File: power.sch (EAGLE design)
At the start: 29 parts, among them CN1 21700, CN2 21700, CN3 21700, CN5 15PIN 0.5MM, Q1 SIRA36DP-T1-GE3, Q2 SIRA36DP-T1-GE3, U1 MAX17320G20+

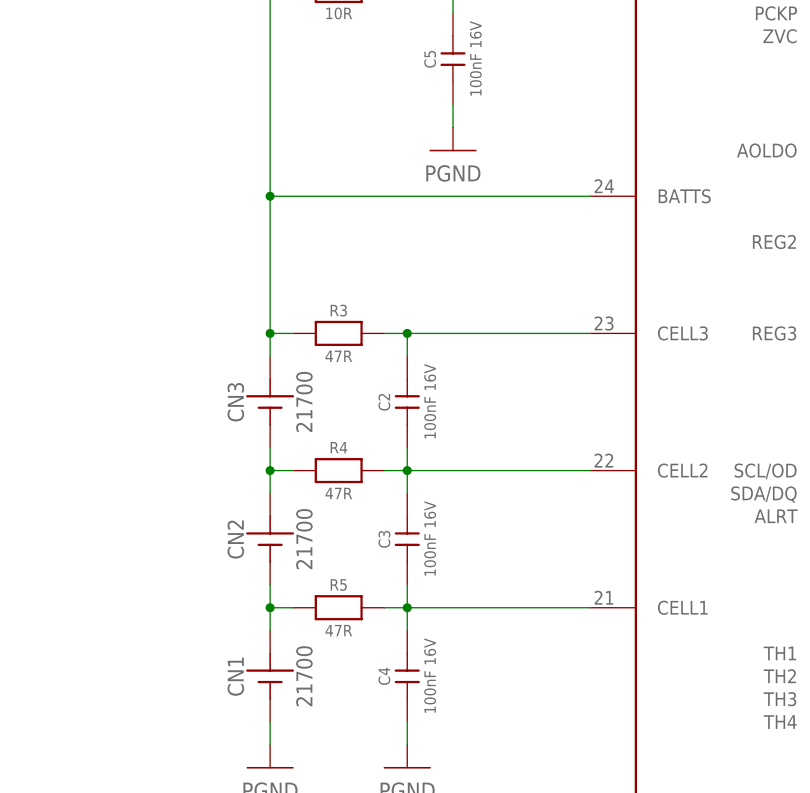
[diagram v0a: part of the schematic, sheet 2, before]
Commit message: Passing DRC
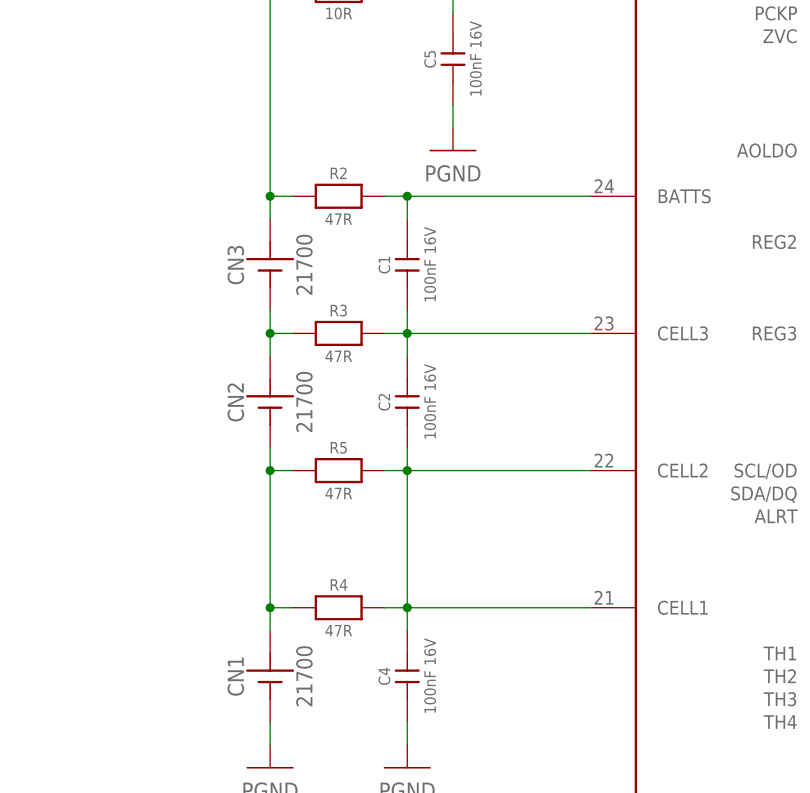
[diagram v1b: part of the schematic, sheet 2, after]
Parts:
- removed C3: 100nF 16V, CAPACITORS:CL10B104KO8WPNC
- added C1: 100nF 16V, CAPACITORS:CL10B104KO8WPNC
- added R2: 47R, r_0603:ERJ3EKF47R0V
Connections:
- removed net N$5: CN2.V+, CN3.V-, R4.1
- new net N$4: CN2.V+, CN3.V-, R3.1
- net N$1: now also C1.2, R2.2, U1.BATTS; no longer C3.1, C4.2, R5.2, U1.CELL1
- net N$2: now also C1.1
- net N$3: now also C4.2, R5.2, U1.CELL1; no longer C3.2
- net N$39: now also R2.1; no longer R3.1, U1.BATTS
- net PACK_MID: now also R4.1
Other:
- moved on the sheet: CN2, CN3, R4, R5
